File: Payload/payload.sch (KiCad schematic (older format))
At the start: 40 parts

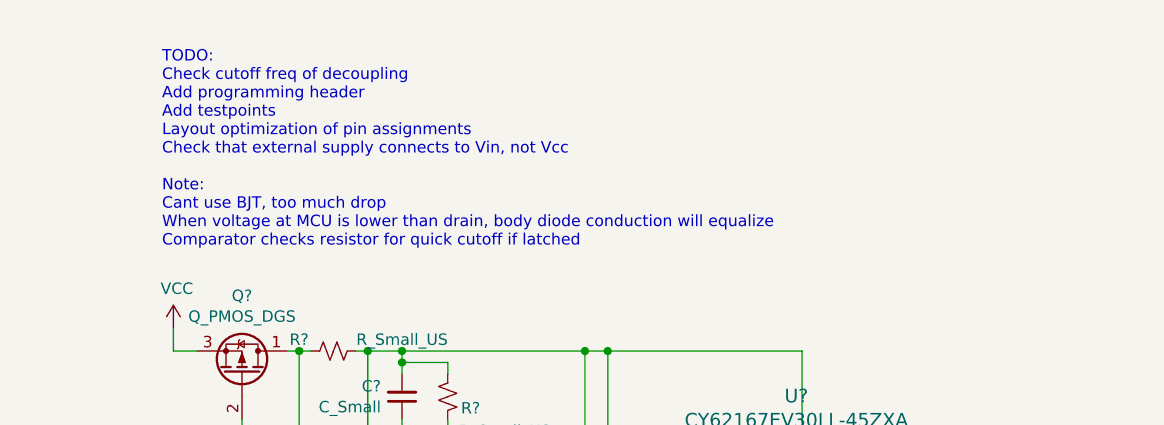
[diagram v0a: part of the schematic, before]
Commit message: Add additional TODO
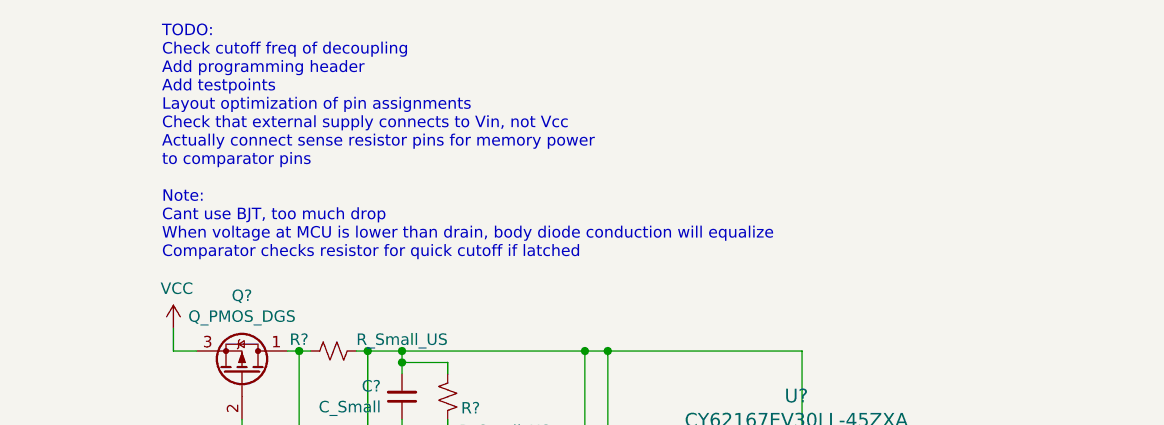
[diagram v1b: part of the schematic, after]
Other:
- note added: "TODO:\nCheck cutoff freq of decoupling\nAdd programming header\nAdd testpoints\nLayout optimization of pin assignments\nCheck that external supply connects to Vin, not Vcc\nActually connect sense resistor pins for memory power\nto comparator pins\n\nNote:\nCant use BJT, too much drop\nWhen voltage at MCU is lower than drain, body diode conduction will equalize\nComparator checks resistor for quic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"
- note removed: "TODO:\nCheck cutoff freq of decoupling\nAdd programming header\nAdd testpoints\nLayout optimization of pin assignments\nCheck that external supply connects to Vin, not Vcc\n\nNote:\nCant use BJT, too much drop\nWhen voltage at MCU is lower than drain, body diode conduction will equalize\nComparator checks resistor for quick cutoff if latched"
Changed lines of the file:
@@
 Wire Wire Line
 	6350 2250 6350 2350
-Text Notes 6000 1500 0    50   ~ 0
-TODO:\nCheck cutoff freq of decoupling\nAdd programming header\nAdd testpoints\nLayout optimization of pin assignments\nCheck that external supply connects to Vin, not Vcc\n\nNote:\nCant use BJT, too much drop\nWhen voltage at MCU is lower than drain, body diode conduction will equalize\nComparator checks resistor for quick cutoff if latched
+Text Notes 6000 1550 0    50   ~ 0
+TODO:\nCheck cutoff freq of decoupling\nAdd programming header\nAdd testpoints\nLayout optimization of pin assignments\nCheck that external supply connects to Vin, not Vcc\nActually connect sense resistor pins for memory power\nto comparator pins\n\nNote:\nCant use BJT, too much drop\nWhen voltage at MCU is lower than drain, body diode conduction will equalize\nComparator checks resistor for quick cutoff if latched
 Wire Wire Line
 	8750 5050 8750 5100
